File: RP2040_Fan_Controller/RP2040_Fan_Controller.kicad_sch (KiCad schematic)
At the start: 19 parts

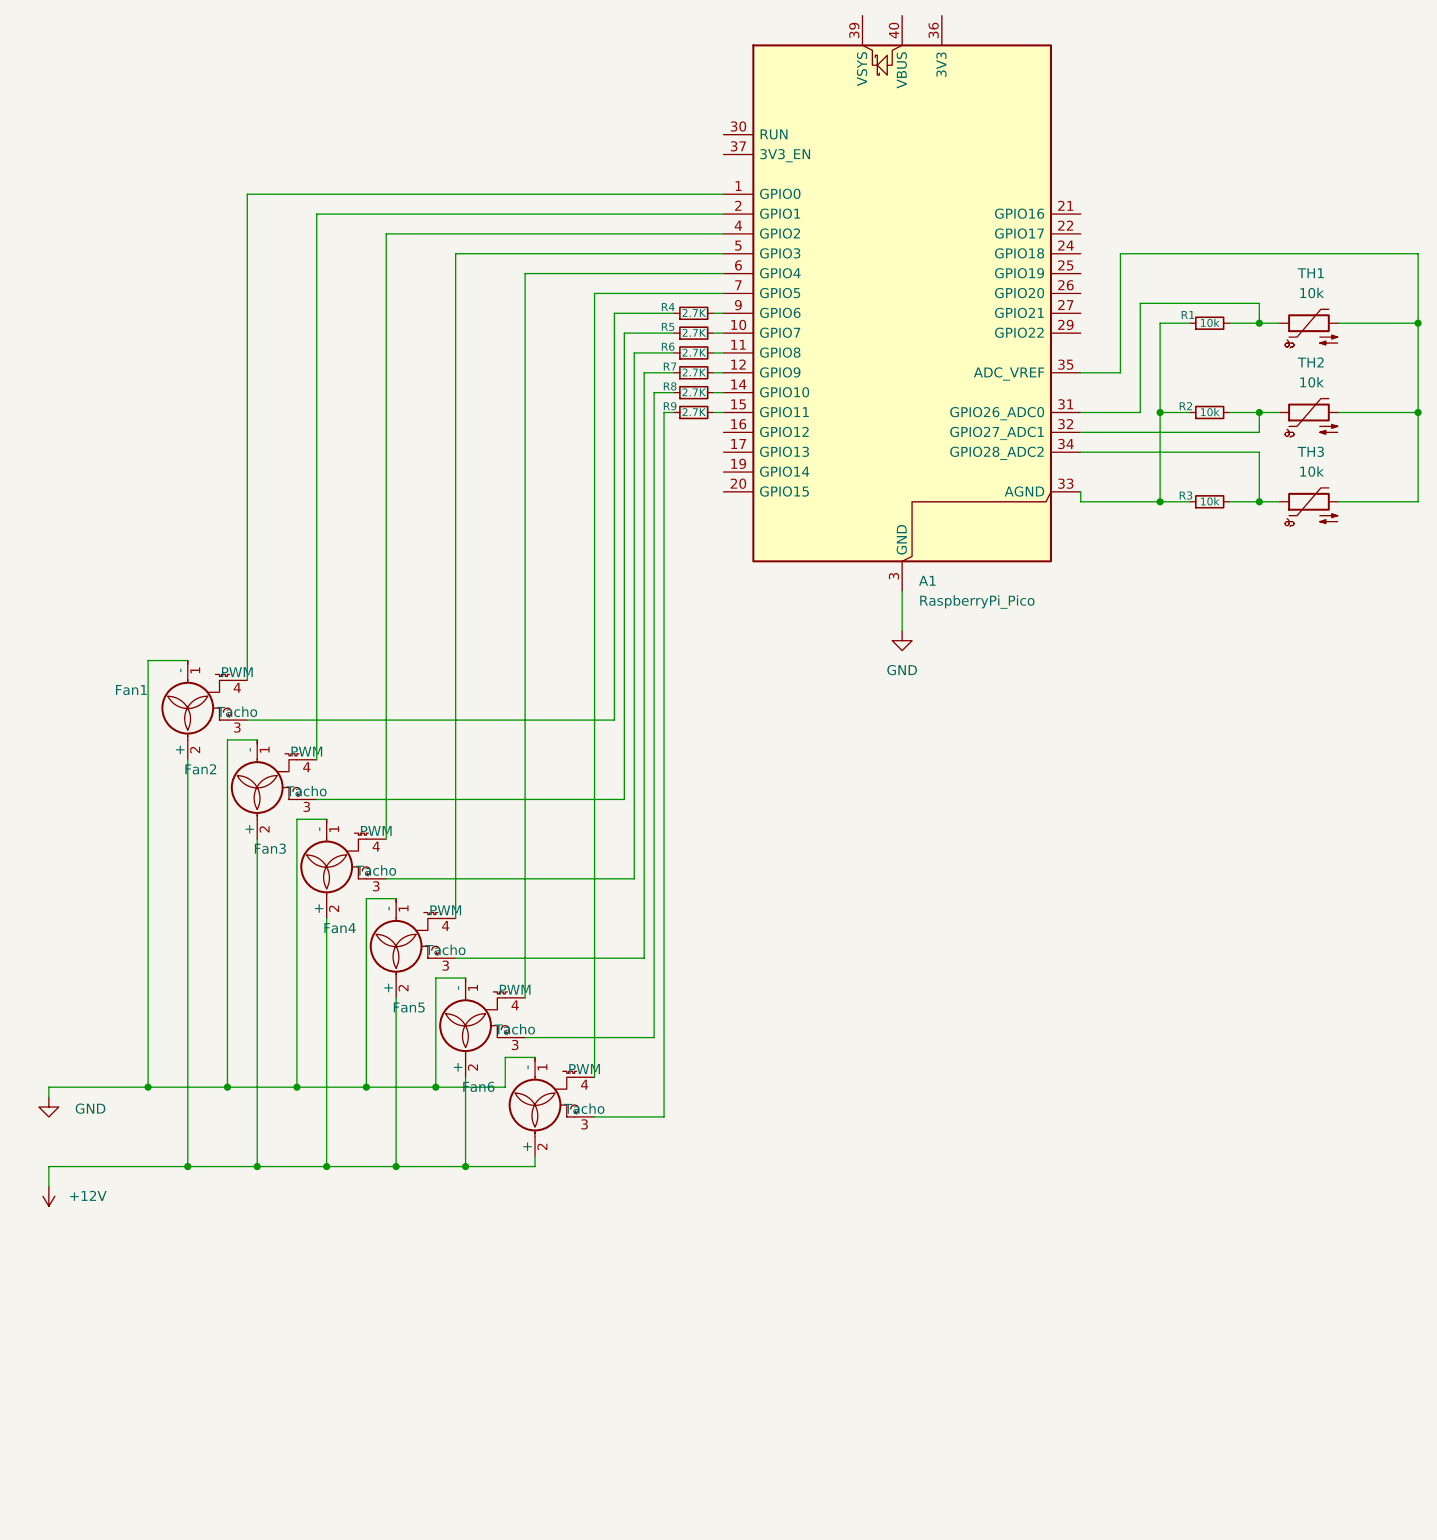
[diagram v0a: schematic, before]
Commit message: PCB-Rev 0.4.0
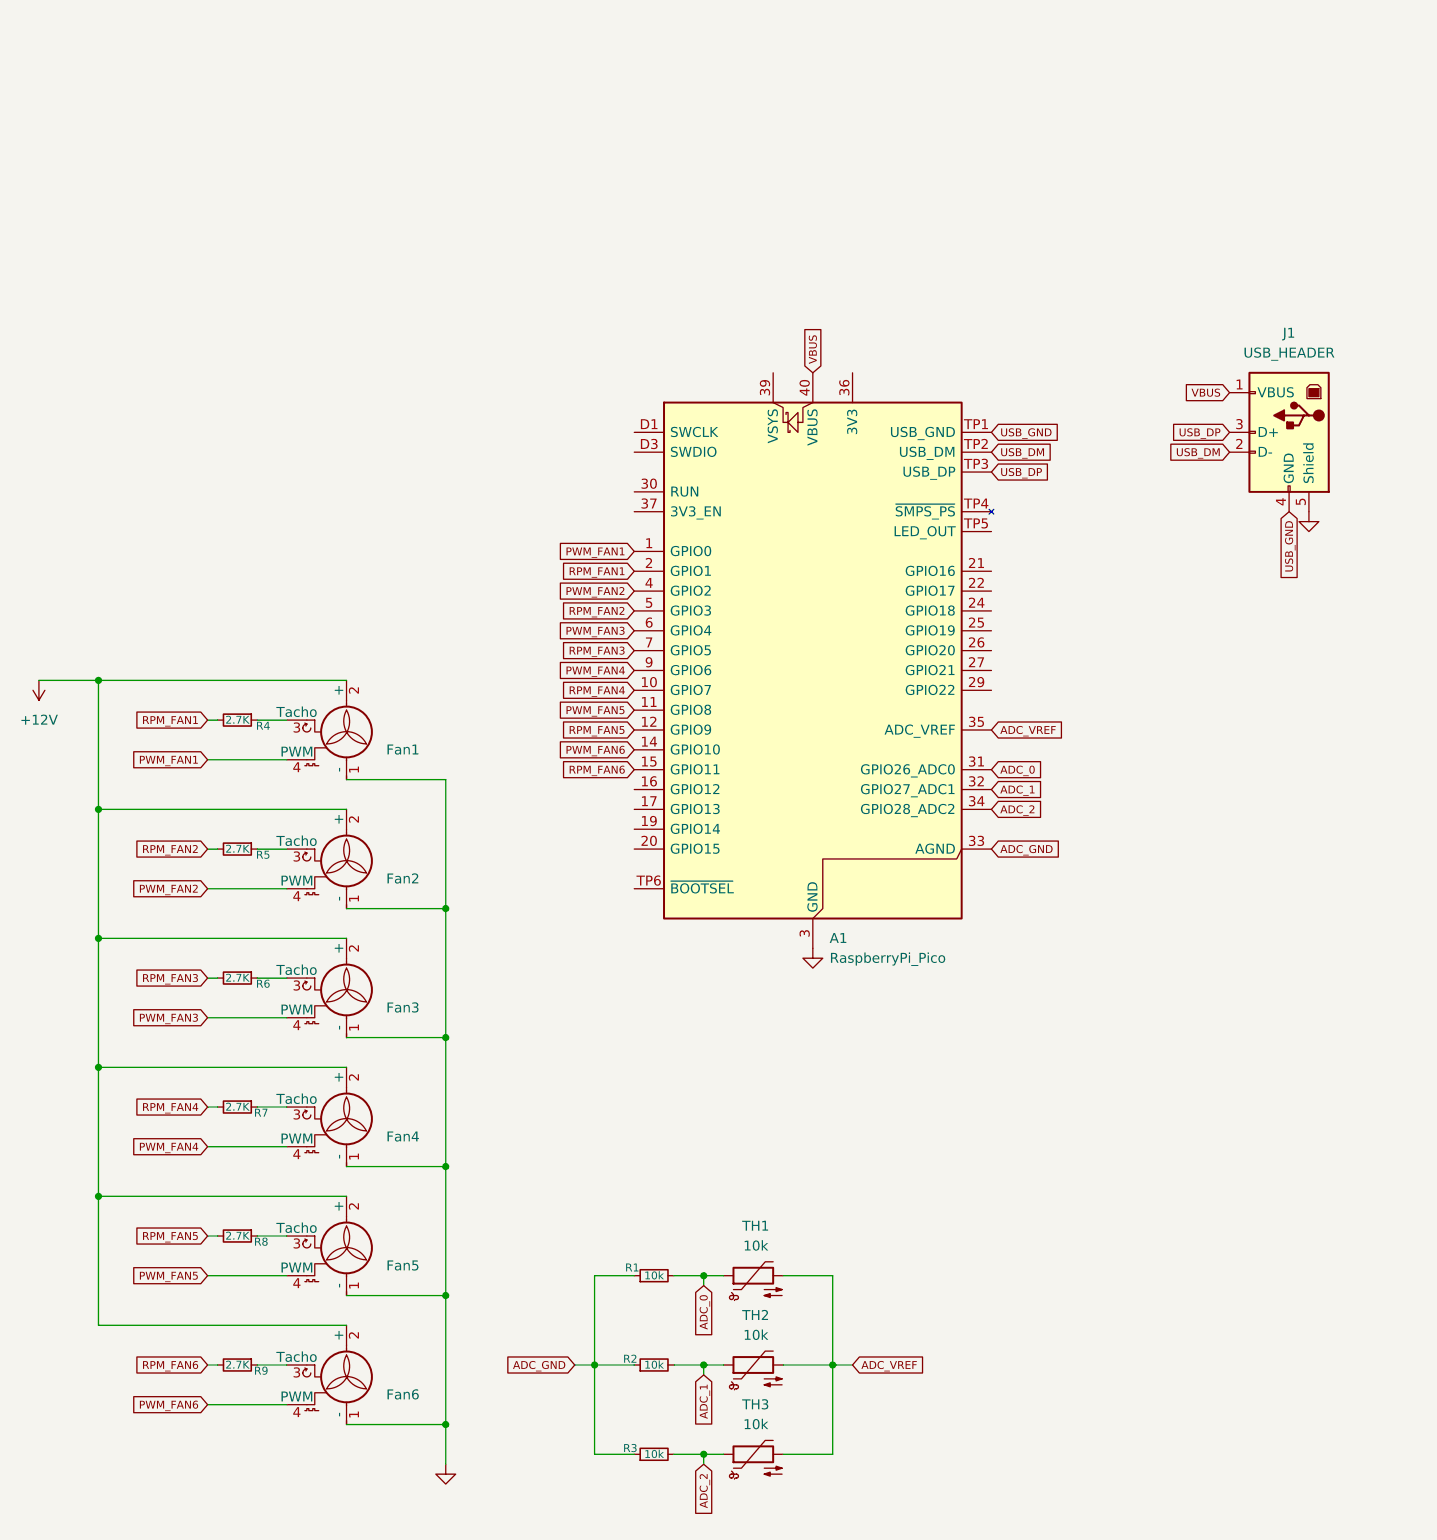
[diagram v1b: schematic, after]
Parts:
- removed A1: RaspberryPi_Pico, Module:RaspberryPi_Pico_Common_Unspecified, symbol MCU_Module:RaspberryPi_Pico
- added A1: RaspberryPi_Pico, Module:RaspberryPi_Pico_SMD, symbol MCU_Module:RaspberryPi_Pico_Extensive
- added J1: USB_HEADER, Connector_PinHeader_2.54mm:PinHeader_1x05_P2.54mm_Horizontal, symbol Connector:USB_B
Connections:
- net GND: now also A1.13 (GND), A1.18 (GND), A1.23 (GND), A1.28 (GND), A1.3 (GND), A1.38 (GND), A1.8 (GND), A1.D2 (GND), J1.5 (Shield)
- net RPM_FAN4: now reaches R7.2
- net RPM_FAN4: now also A1.10 (GPIO7)
- net PWM_FAN1: now reaches Fan1.4 (PWM)
- net PWM_FAN1: now also A1.1 (GPIO0)
- net PWM_FAN5: now reaches Fan5.4 (PWM)
- net PWM_FAN5: now also A1.11 (GPIO8)
- net RPM_FAN2: now reaches R5.2
- net RPM_FAN2: now also A1.5 (GPIO3)
- net RPM_FAN3: now reaches R6.2
- net RPM_FAN3: now also A1.7 (GPIO5)
- net RPM_FAN5: now reaches R8.2
- net RPM_FAN5: now also A1.12 (GPIO9)
- net RPM_FAN6: now reaches R9.2
- net RPM_FAN6: now also A1.15 (GPIO11)
- net PWM_FAN2: now reaches Fan2.4 (PWM)
- net PWM_FAN2: now also A1.4 (GPIO2)
- net ADC_0: now reaches R1.2, TH1.1
- net ADC_0: now also A1.31 (GPIO26_ADC0)
- net ADC_1: now reaches R2.2, TH2.1
- net ADC_1: now also A1.32 (GPIO27_ADC1)
- net ADC_GND: now reaches R1.1, R2.1, R3.1
- net ADC_GND: now also A1.33 (AGND)
- net ADC_2: now reaches R3.2, TH3.1
- net ADC_2: now also A1.34 (GPIO28_ADC2)
- net ADC_VREF: now reaches TH1.2, TH2.2, TH3.2
- net ADC_VREF: now also A1.35 (ADC_VREF)
- net PWM_FAN3: now reaches Fan3.4 (PWM)
- net PWM_FAN3: now also A1.6 (GPIO4)
- net PWM_FAN4: now reaches Fan4.4 (PWM)
- net PWM_FAN4: now also A1.9 (GPIO6)
- net PWM_FAN6: now reaches Fan6.4 (PWM)
- net PWM_FAN6: now also A1.14 (GPIO10)
- net RPM_FAN1: now reaches R4.2
- net RPM_FAN1: now also A1.2 (GPIO1)
- new net USB_DM: A1.TP2 (USB_DM), J1.2 (D-)
- new net USB_DP: A1.TP3 (USB_DP), J1.3 (D+)
- new net USB_GND: A1.TP1 (USB_GND), J1.4 (GND)
- new net VBUS: A1.40 (VBUS), J1.1 (VBUS)
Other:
- moved on the sheet: Fan1, Fan2, Fan3, Fan4, Fan5, Fan6, R1, R2, R3, R4, R5, R6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
